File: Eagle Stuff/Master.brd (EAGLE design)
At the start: 160 x 100 mm, 5 parts

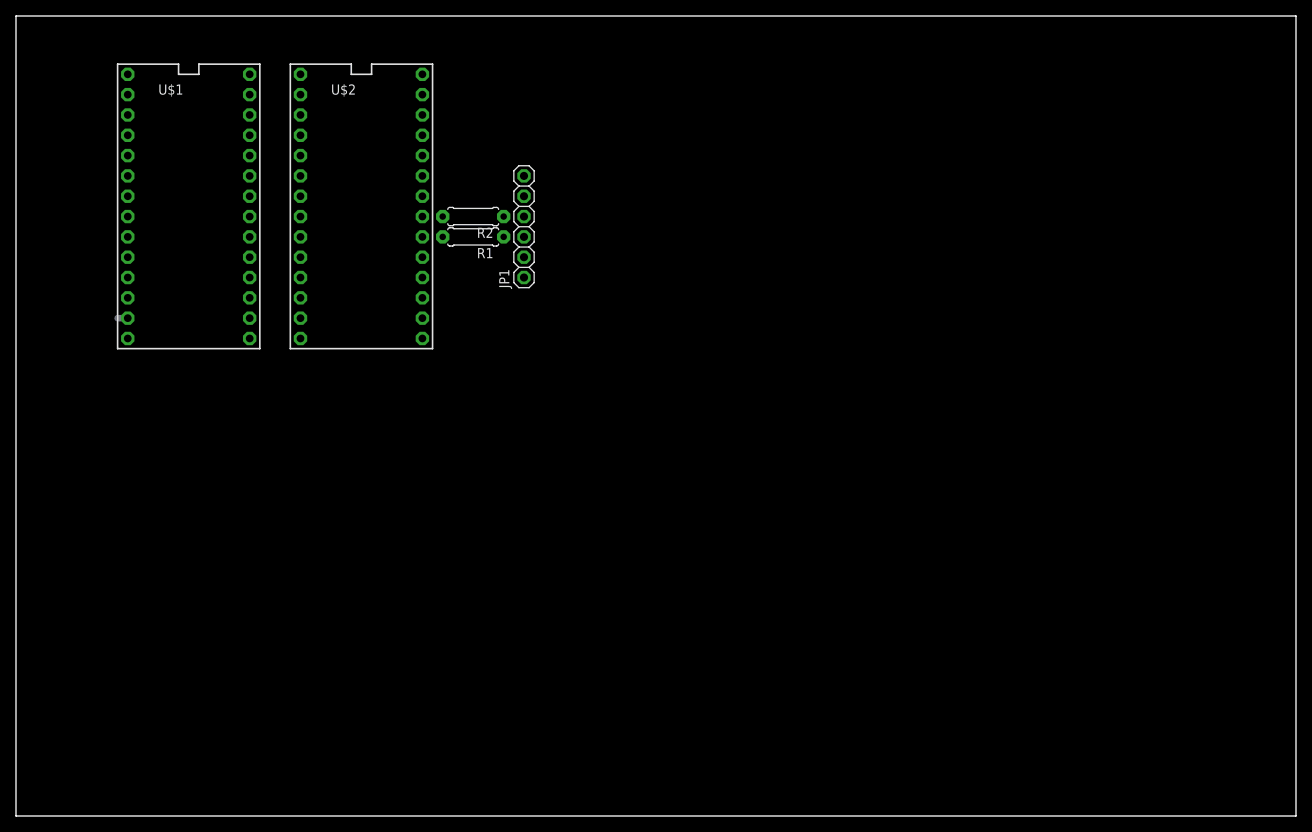
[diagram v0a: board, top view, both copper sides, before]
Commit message: Initial commit for master board
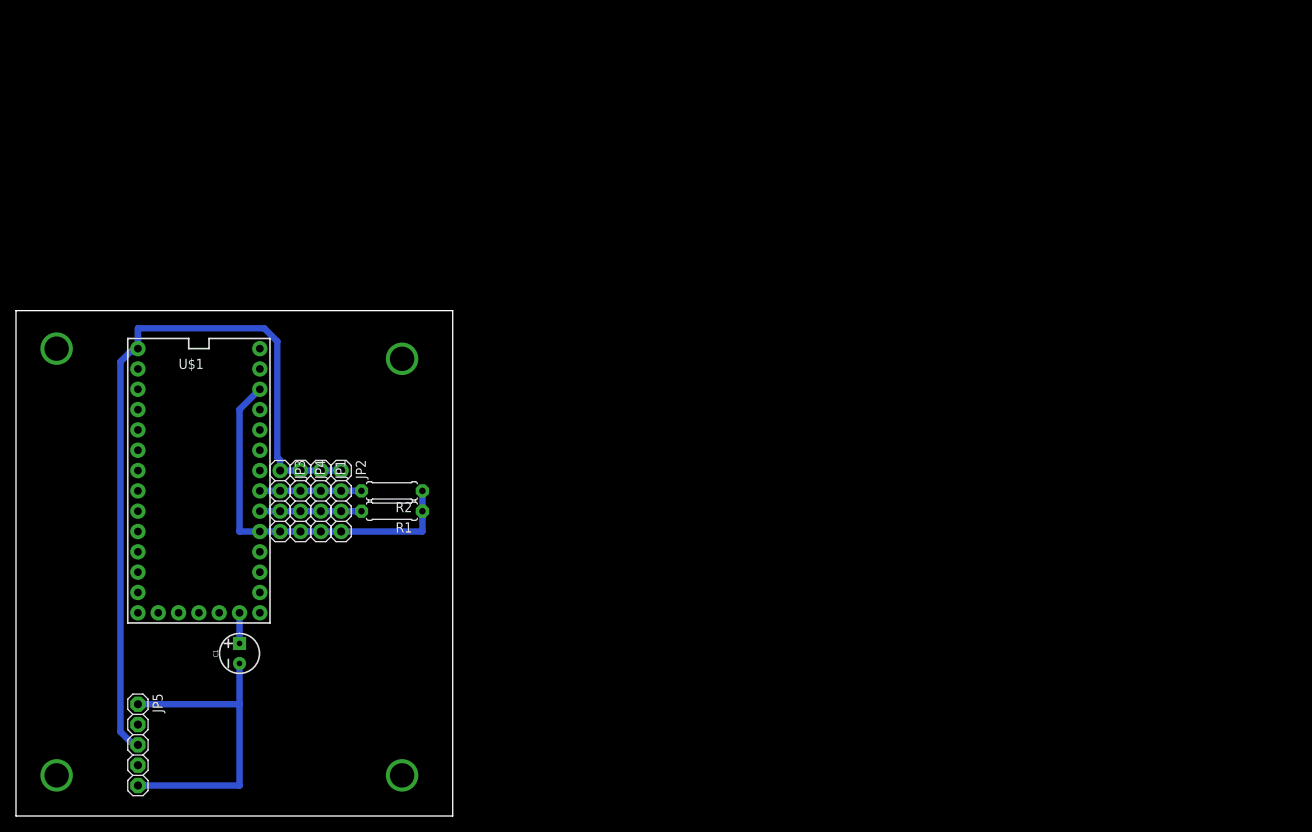
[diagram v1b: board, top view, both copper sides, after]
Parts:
- removed U$2: TEENSY_3.1-3.2_DIL, Teensy_3_and_LC_Series_Boards_v1.4:TEENSY_3.0-3.2&LC_DIL
- added C1: 10uF, SparkFun-Capacitors:CPOL-RADIAL-2.5MM-5MM
- added JP2, JP3, JP4: (no value), pinhead:1X04
- added JP5: (no value), pinhead:1X05
- JP1: device pinhead:1X06 -> pinhead:1X04
- U$1: value TEENSY_3.1-3.2_DIL -> TEENSY_3.1-3.2_OUTER_ROW; device Teensy_3_and_LC_Series_Boards_v1.4:TEENSY_3.0-3.2&LC_DIL -> Teensy_3_and_LC_Series_Boards_v1.4:TEENSY_3.0-3.2&LC_OUTER_ROW
- moved JP1 42.7 mm to (38.1, 39.4), turned to 270 degrees
- moved R2 35.8 mm to (47.0, 40.6)
- moved R1 35.8 mm to (47.0, 38.1)
- moved U$1 34.3 mm to (22.9, 41.9)
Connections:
- removed net N$10: U$1.6, U$2.6
- removed net N$11: U$1.13, U$2.13
- removed net N$12: U$1.14/A0, U$2.14/A0
- removed net N$13: U$1.15/A1, U$2.15/A1
- removed net N$14: U$1.23/A9, U$2.23/A9
- removed net N$15: U$1.22/A8, U$2.22/A8
- removed net N$5: U$1.11, U$2.11
- removed net N$6: U$1.12, U$2.12
- removed net N$7: U$1.10, U$2.10
- removed net N$8: U$1.9, U$2.9
- removed net N$9: U$1.7, U$2.7
- new net N$1: JP1.3, JP2.3, JP3.3, JP4.3, R1.2, U$1.18/A4
- new net N$4: C1.2, JP5.1, JP5.5
- new net VBAT: U$1.VBAT
- net AGND: no longer U$2.AGND
- net GND: now also JP1.1, JP2.1, JP3.1, JP4.1, JP5.3, U$1.GND1; no longer JP1.6, U$2.GND
- net N$2: now also JP1.2, JP2.2, JP3.2, JP4.2, R2.2, U$1.19/A5; no longer JP1.3, R1.2, U$1.18/A4, U$2.18/A4
- net N$3: now also C1.1, U$1.RESET/DAC; no longer JP1.4, R2.2, U$1.19/A5, U$2.19/A5
- net VCC: now also JP1.4, JP2.4, JP3.4, JP4.4, U$1.3.3V1; no longer JP1.1, U$2.3.3V
- net VIN: no longer U$2.VIN
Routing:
- net GND: track 0.00 -> 96.5 mm
- net VCC: track 0.00 -> 46.8 mm
- net N$4: track 0.00 -> 40.7 mm
- net N$2: track 0.00 -> 12.7 mm
- net N$1: track 0.00 -> 12.7 mm
- net N$3: track 0.00 -> 3.83 mm
- net N$5: track 1.27 -> 0.00 mm, vias 0 -> 1
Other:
- board size 160 x 100 mm -> 54.6 x 63.2 mm
